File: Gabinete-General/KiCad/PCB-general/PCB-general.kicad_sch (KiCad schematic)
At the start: 14 parts, among them J1 Conn_01x02, J2 Conn_01x02, J3 TFT Display, J4 PCIe X4, SW1 RotaryEncoder_Switch, U1 ESP32-S3-DevKitC, U2 LM7805_TO220

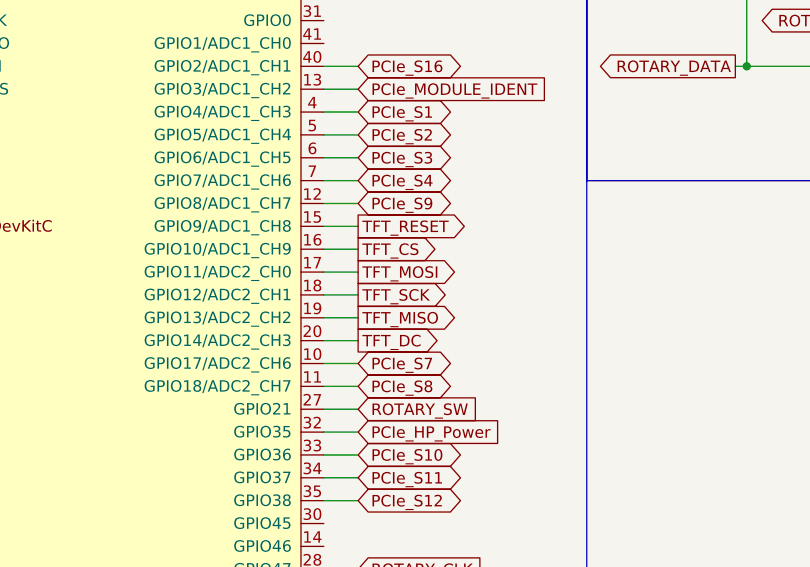
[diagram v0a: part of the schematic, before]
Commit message: Diseño inicial PCB
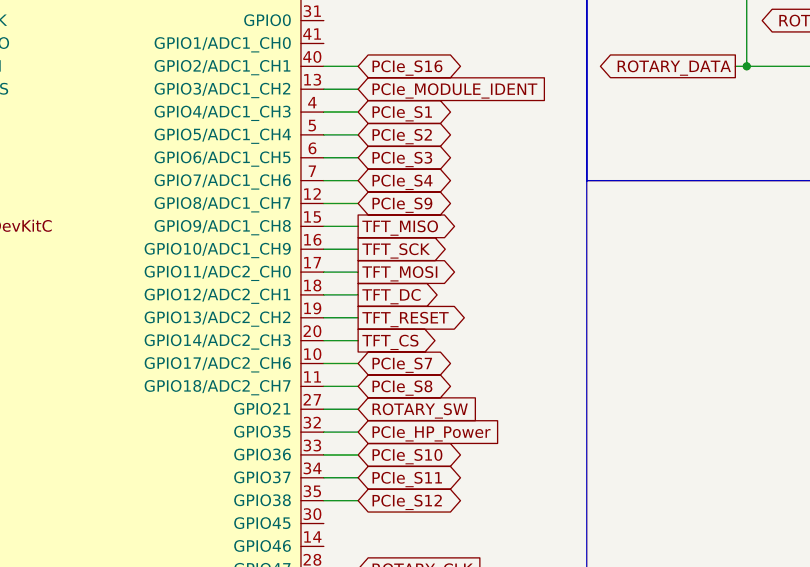
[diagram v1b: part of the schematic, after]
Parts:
- SW1: footprint Rotary_Encoder:RotaryEncoder_Alps_EC11E-Switch_Vertical_H20mm -> Connector_PinHeader_2.54mm:PinHeader_1x05_P2.54mm_Vertical
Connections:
- net TFT_CS: now also U1.20 (GPIO14/ADC2_CH3); no longer U1.16 (GPIO10/ADC1_CH9)
- net TFT_DC: now also U1.18 (GPIO12/ADC2_CH1); no longer U1.20 (GPIO14/ADC2_CH3)
- net TFT_MISO: now also U1.15 (GPIO9/ADC1_CH8); no longer U1.19 (GPIO13/ADC2_CH2)
- net TFT_RESET: now also U1.19 (GPIO13/ADC2_CH2); no longer U1.15 (GPIO9/ADC1_CH8)
- net TFT_SCK: now also U1.16 (GPIO10/ADC1_CH9); no longer U1.18 (GPIO12/ADC2_CH1)
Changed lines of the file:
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@@
 	(wire
 		(pts
+			(xy 96.52 119.38) (xy 92.71 119.38)
+		)
+		(stroke
+			(width 0)
+			(type default)
+		)
+	)
+	(wire
+		(pts
 			(xy 96.52 147.32) (xy 92.71 147.32)
 		)
@@
 	(wire
 		(pts
-			(xy 92.71 114.3) (xy 96.52 114.3)
-		)
-		(stroke
-			(width 0)
-			(type default)
-		)
-	)
-	(wire
-		(pts
 			(xy 92.71 104.14) (xy 96.52 104.14)
 		)
@@
 	(wire
 		(pts
-			(xy 139.7 82.55) (xy 139.7 91.44)
+			(xy 96.52 109.22) (xy 92.71 109.22)
 		)
 		(stroke
@@
 	(wire
 		(pts
-			(xy 92.71 111.76) (xy 96.52 111.76)
+			(xy 139.7 82.55) (xy 139.7 91.44)
 		)
 		(stroke
@@
 	(wire
 		(pts
-			(xy 92.71 109.22) (xy 96.52 109.22)
-		)
-		(stroke
-			(width 0)
-			(type default)
-		)
-	)
-	(wire
-		(pts
-			(xy 92.71 119.38) (xy 96.52 119.38)
-		)
-		(stroke
-			(width 0)
-			(type default)
-		)
-	)
-	(wire
-		(pts
 			(xy 96.52 149.86) (xy 92.71 149.86)
 		)
@@
 	(wire
 		(pts
+			(xy 96.52 121.92) (xy 92.71 121.92)
+		)
+		(stroke
+			(width 0)
+			(type default)
+		)
+	)
+	(wire
+		(pts
 			(xy 138.43 91.44) (xy 139.7 91.44)
 		)
@@
 	(wire
 		(pts
-			(xy 92.71 121.92) (xy 96.52 121.92)
-		)
-		(stroke
-			(width 0)
-			(type default)
-		)
-	)
-	(wire
-		(pts
 			(xy 179.07 86.36) (xy 182.88 86.36)
 		)
@@
 	(wire
 		(pts
-			(xy 92.71 116.84) (xy 96.52 116.84)
+			(xy 218.44 63.5) (xy 222.25 63.5)
 		)
 		(stroke
@@
 	(wire
 		(pts
-			(xy 218.44 63.5) (xy 222.25 63.5)
+			(xy 156.21 74.93) (xy 179.07 74.93)
 		)
 		(stroke
@@
 	(wire
 		(pts
-			(xy 156.21 74.93) (xy 179.07 74.93)
+			(xy 252.73 63.5) (xy 256.54 63.5)
 		)
 		(stroke
@@
 	(wire
 		(pts
-			(xy 252.73 63.5) (xy 256.54 63.5)
+			(xy 252.73 68.58) (xy 256.54 68.58)
 		)
 		(stroke
@@
 	(wire
 		(pts
-			(xy 252.73 68.58) (xy 256.54 68.58)
+			(xy 180.34 45.72) (xy 180.34 46.99)
 		)
 		(stroke
@@
 	(wire
 		(pts
-			(xy 180.34 45.72) (xy 180.34 46.99)
+			(xy 180.34 53.34) (xy 180.34 67.31)
 		)
 		(stroke
@@
 	(wire
 		(pts
-			(xy 180.34 53.34) (xy 180.34 67.31)
+			(xy 69.85 44.45) (xy 69.85 45.72)
 		)
 		(stroke
@@
 	(wire
 		(pts
-			(xy 69.85 44.45) (xy 69.85 45.72)
+			(xy 96.52 111.76) (xy 92.71 111.76)
 		)
 		(stroke
@@
 	(wire
 		(pts
+			(xy 96.52 114.3) (xy 92.71 114.3)
+		)
+		(stroke
+			(width 0)
+			(type default)
+		)
+	)
+	(wire
+		(pts
 			(xy 92.71 139.7) (xy 96.52 139.7)
 		)
@@
 	(wire
 		(pts
+			(xy 96.52 116.84) (xy 92.71 116.84)
+		)
+		(stroke
+			(width 0)
+			(type default)
+		)
+	)
+	(wire
+		(pts
 			(xy 194.31 45.72) (xy 180.34 45.72)
 		)
@@
 	(global_label "TFT_MISO"
 		(shape output)
-		(at 96.52 119.38 0)
+		(at 96.52 109.22 0)
 		(fields_autoplaced yes)
 		(effects
@@
 		)
 		(property "Intersheetrefs" "${INTERSHEET_REFS}"
-			(at 108.0928 119.38 0)
+			(at 108.0928 109.22 0)
 			(effects
 				(font
@@
 	(global_label "TFT_RESET"
 		(shape output)
-		(at 96.52 109.22 0)
+		(at 96.52 119.38 0)
 		(fields_autoplaced yes)
 		(effects
@@
 		)
 		(property "Intersheetrefs" "${INTERSHEET_REFS}"
-			(at 109.2417 109.22 0)
+			(at 109.2417 119.38 0)
 			(effects
 				(font
@@
 	(global_label "TFT_DC"
 		(shape output)
-		(at 96.52 121.92 0)
+		(at 96.52 116.84 0)
 		(fields_autoplaced yes)
 		(effects
@@
 		)
 		(property "Intersheetrefs" "${INTERSHEET_REFS}"
-			(at 106.0366 121.92 0)
+			(at 106.0366 116.84 0)
 			(effects
 				(font
@@
 	(global_label "TFT_CS"
 		(shape output)
-		(at 96.52 111.76 0)
+		(at 96.52 121.92 0)
 		(fields_autoplaced yes)
 		(effects
@@
 		)
 		(property "Intersheetrefs" "${INTERSHEET_REFS}"
-			(at 105.9761 111.76 0)
+			(at 105.9761 121.92 0)
 			(effects
 				(font
@@
 	(global_label "TFT_SCK"
 		(shape output)
-		(at 96.52 116.84 0)
+		(at 96.52 111.76 0)
 		(fields_autoplaced yes)
 		(effects
@@
 		)
 		(property "Intersheetrefs" "${INTERSHEET_REFS}"
-			(at 107.2461 116.84 0)
+			(at 107.2461 111.76 0)
 			(effects
 				(font
@@
 			)
 		)
-		(property "Footprint" "Rotary_Encoder:RotaryEncoder_Alps_EC11E-Switch_Vertical_H20mm"
+		(property "Footprint" "Connector_PinHeader_2.54mm:PinHeader_1x05_P2.54mm_Vertical"
 			(at 163.83 84.836 0)
 			(effects
